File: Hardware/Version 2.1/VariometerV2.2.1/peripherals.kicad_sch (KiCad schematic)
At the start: 23 parts, among them J1 USB_C_Receptacle_USB2.0, J2 Conn_01x02, J3 Conn_01x02, J4 Conn_01x02, J5 Conn_01x02, J6 Conn_01x02, J7 Conn_01x02, U1 SRV05-4

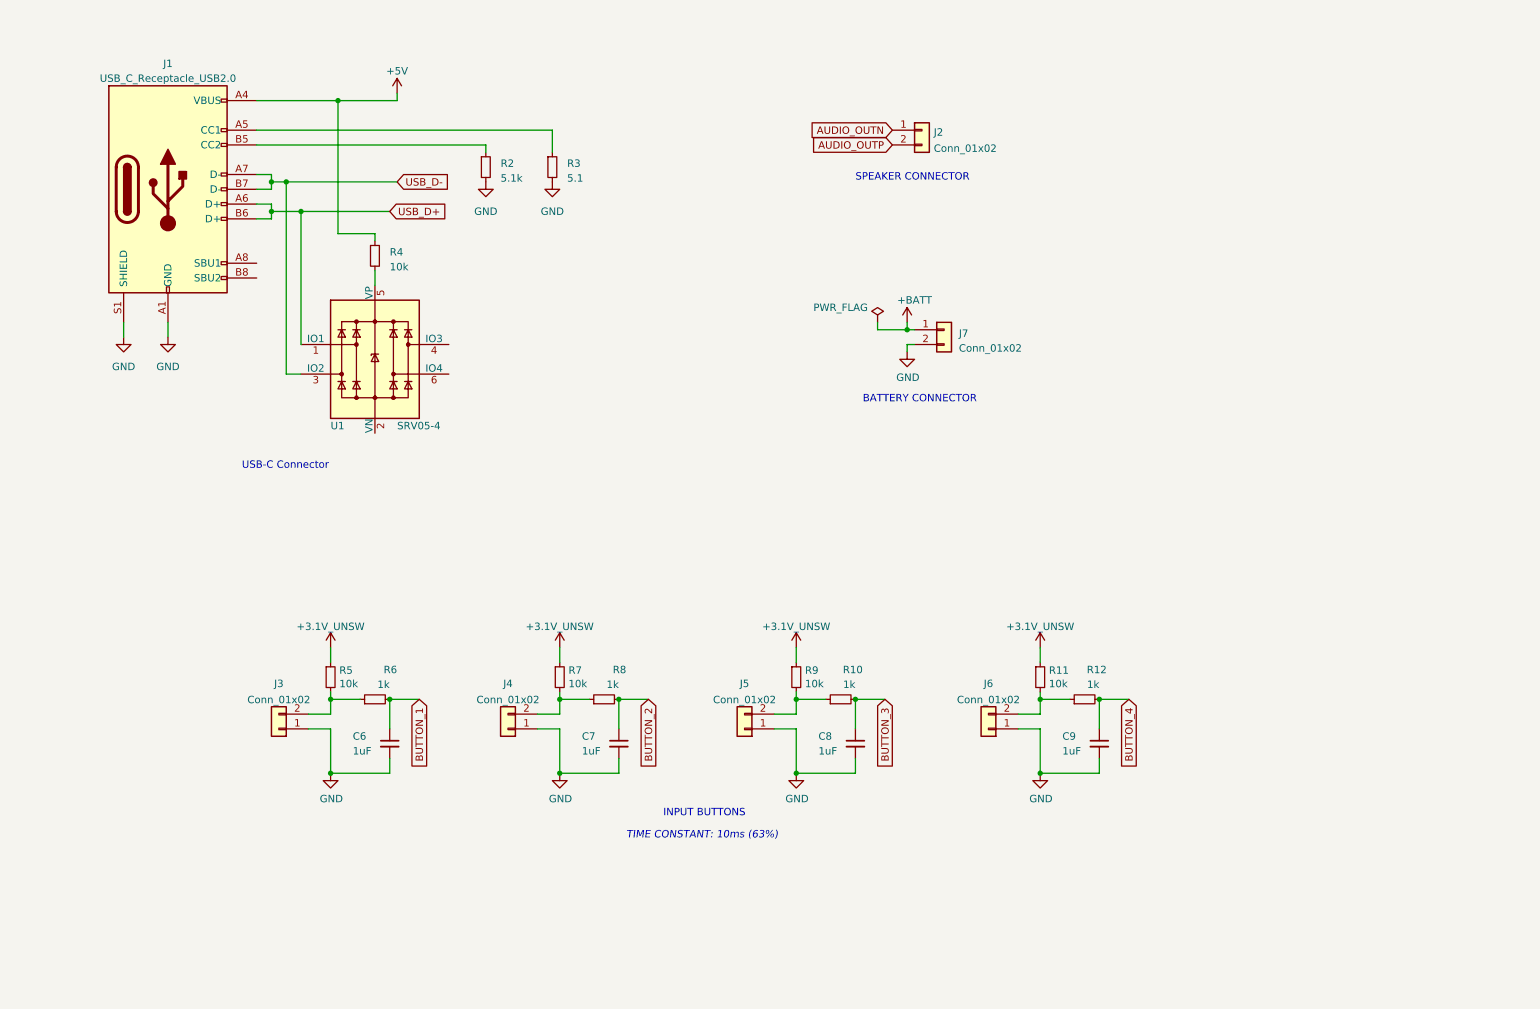
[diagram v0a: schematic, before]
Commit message: Working on PCB
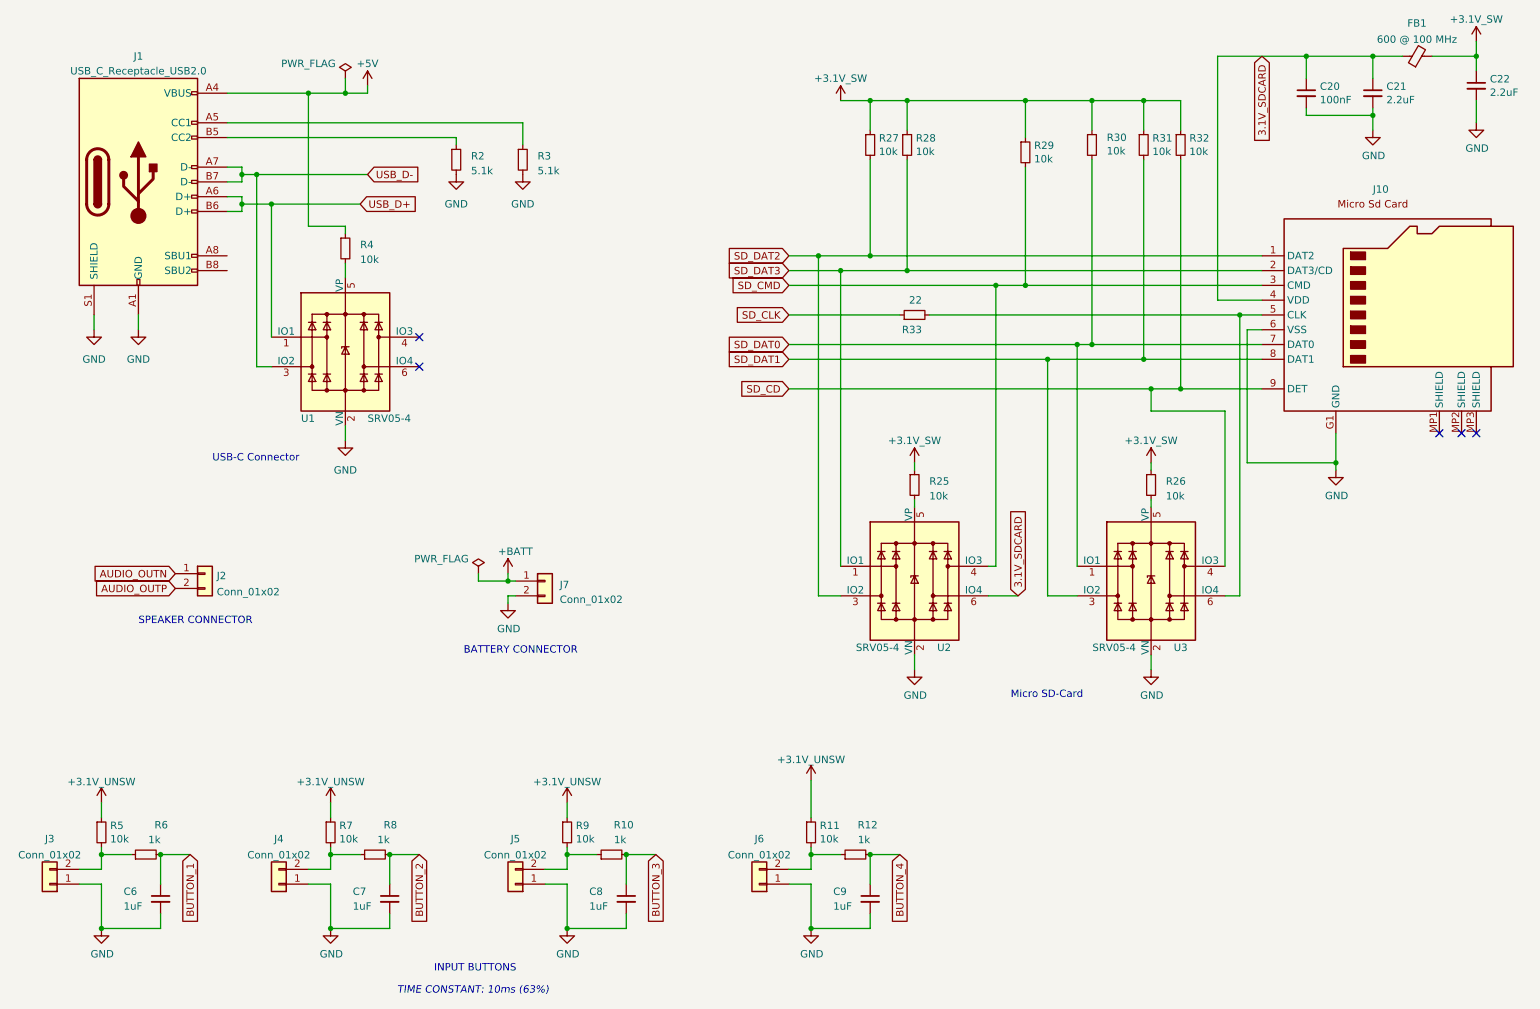
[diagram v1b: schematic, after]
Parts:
- added C20: 100nF, Capacitor_SMD:C_0402_1005Metric, symbol Device:C_Small
- added C21, C22: 2.2uF, Capacitor_SMD:C_0603_1608Metric, symbol Device:C_Small
- added FB1: 600 @ 100 MHz, Inductor_SMD:L_0603_1608Metric, symbol Device:FerriteBead_Small
- added J10: ~, symbol Main_LibraryVario:Micro_SD_Card
- added R25, R26: 10k, symbol Device:R_Small
- added R27, R28, R29, R30, R31, R32: 10k, Resistor_SMD:R_0402_1005Metric, symbol Device:R_Small
- added R33: 22, Resistor_SMD:R_0402_1005Metric, symbol Device:R_Small
- added U2, U3: SRV05-4, Package_TO_SOT_SMD:SOT-23-6, symbol Power_Protection:SRV05-4
- R3: value 5.1 -> 5.1k
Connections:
- net GND: now also U1.2 (VN), C20.2, C21.2, C22.2, J10.6 (VSS), J10.G1 (GND), U2.2 (VN), U3.2 (VN)
- new net: J10.5 (CLK), R33.2, U3.6 (IO4)
- new net: R26.2, U3.5 (VP)
- new net: R25.2, U2.5 (VP)
- new net +3.1V_SW: C22.1, FB1.2, R25.1, R26.1, R27.1, R28.1, R29.1, R30.1, R31.1, R32.1
- new net 3.1V_SDCARD: C20.1, C21.1, FB1.1, J10.4 (VDD), U2.6 (IO4)
- new net SD_CD: J10.9 (DET), R32.2, U3.4 (IO3)
- new net SD_CLK: R33.1
- new net SD_CMD: J10.3 (CMD), R29.2, U2.4 (IO3)
- new net SD_DAT0: J10.7 (DAT0), R30.2, U3.1 (IO1)
- new net SD_DAT1: J10.8 (DAT1), R31.2, U3.3 (IO2)
- new net SD_DAT2: J10.1 (DAT2), R27.2, U2.3 (IO2)
- new net SD_DAT3: J10.2 (DAT3/CD), R28.2, U2.1 (IO1)
- no-connect marks 0 -> 5
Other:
- note added: "Micro SD-Card"
- moved on the sheet: C6, C7, C8, C9, J1, J2, J3, J4, J5, J6, J7, R10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
